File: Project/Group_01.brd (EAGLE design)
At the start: 71.1 x 54.3 mm, 29 parts, among them J1 POWER_JACKPTH_LOCK, U1 +12v, U4 TMUX1208

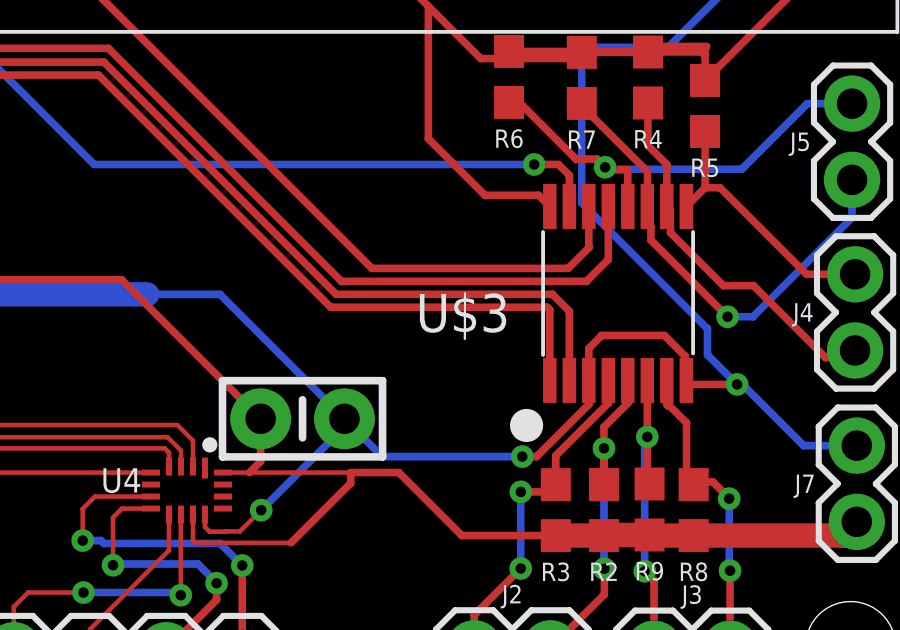
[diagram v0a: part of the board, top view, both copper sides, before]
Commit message: Changed name
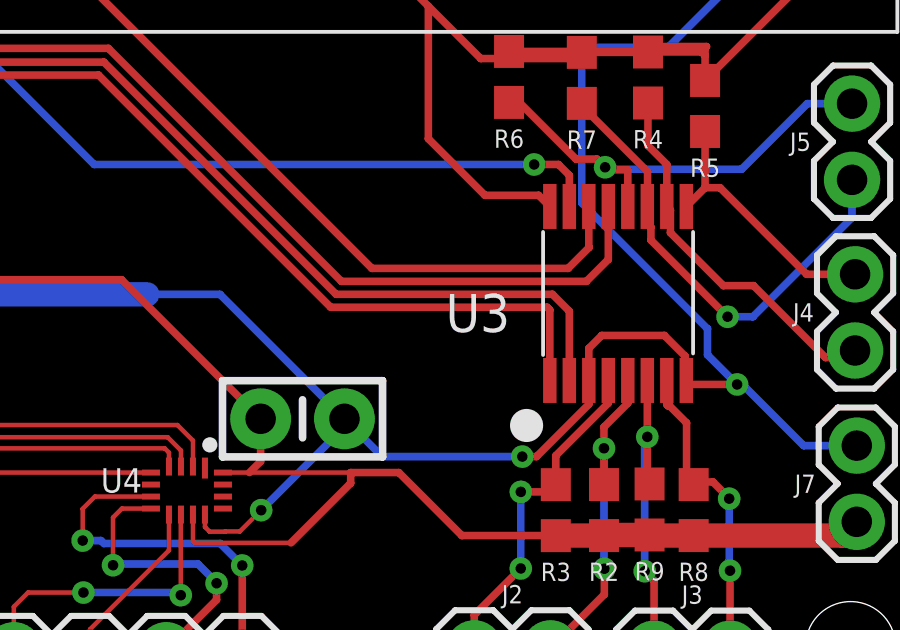
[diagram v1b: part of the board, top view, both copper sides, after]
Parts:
- renumbered U$3 to U3
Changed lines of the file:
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@@
 <attribute name="VALUE" x="41.13478125" y="50.174271875" size="0.6096" layer="27" font="vector" ratio="20" rot="R90" align="top-center"/>
 </element>
-<element name="U$3" library="Group_01_Library" package="TSSOP16" value="TCA9546A" x="60.95" y="14.32" smashed="yes" rot="R90">
+<element name="U3" library="Group_01_Library" package="TSSOP16" value="TCA9546A" x="60.95" y="14.32" smashed="yes" rot="R90">
 <attribute name="NAME" x="57.347734375" y="13.668865625" size="1.27" layer="25" align="center-right"/>
 </element>
@@
 <contactref element="C1" pad="2"/>
 <contactref element="U1" pad="3"/>
-<contactref element="U$3" pad="8"/>
-<contactref element="U$3" pad="3"/>
+<contactref element="U3" pad="8"/>
+<contactref element="U3" pad="3"/>
 <contactref element="U$2" pad="28"/>
 <contactref element="R1" pad="P$1"/>
@@
 <contactref element="U1" pad="2"/>
 <contactref element="C1" pad="1"/>
-<contactref element="U$3" pad="16"/>
+<contactref element="U3" pad="16"/>
 <contactref element="R2" pad="2"/>
 <contactref element="R3" pad="2"/>
@@
 </signal>
 <signal name="I2C_SCL_0">
-<contactref element="U$3" pad="5"/>
+<contactref element="U3" pad="5"/>
 <contactref element="R2" pad="1"/>
 <contactref element="J2" pad="2"/>
@@
 <signal name="I2C_SDA_0">
 <contactref element="R3" pad="1"/>
-<contactref element="U$3" pad="4"/>
+<contactref element="U3" pad="4"/>
 <contactref element="J2" pad="1"/>
 <wire x1="60.625" y1="11.42" x2="60.625" y2="10.66395" width="0.254" layer="1"/>
@@
 </signal>
 <signal name="I2C_SDA_1">
-<contactref element="U$3" pad="6"/>
+<contactref element="U3" pad="6"/>
 <contactref element="R9" pad="1"/>
 <contactref element="J3" pad="1"/>
@@
 <signal name="I2C_SCL_1">
 <contactref element="R8" pad="1"/>
-<contactref element="U$3" pad="7"/>
+<contactref element="U3" pad="7"/>
 <contactref element="J3" pad="2"/>
 <wire x1="63.47" y1="7.95" x2="63.2333" y2="8.1867" width="0.254" layer="1"/>
@@
 </signal>
 <signal name="I2C_SDA_2">
-<contactref element="U$3" pad="9"/>
+<contactref element="U3" pad="9"/>
 <contactref element="R5" pad="1"/>
 <contactref element="J4" pad="1"/>
@@
 <signal name="I2C_SCL_2">
 <contactref element="R4" pad="1"/>
-<contactref element="U$3" pad="10"/>
+<contactref element="U3" pad="10"/>
 <contactref element="J4" pad="2"/>
 <wire x1="61.946959375" y1="20.669490625" x2="61.946959375" y2="19.24795" width="0.254" layer="1"/>
@@
 </signal>
 <signal name="I2C_SCL_3">
-<contactref element="U$3" pad="12"/>
+<contactref element="U3" pad="12"/>
 <contactref element="R6" pad="1"/>
 <contactref element="J5" pad="2"/>
@@
 </signal>
 <signal name="I2C_SDA_3">
-<contactref element="U$3" pad="11"/>
+<contactref element="U3" pad="11"/>
 <contactref element="R7" pad="1"/>
 <contactref element="J5" pad="1"/>
@@
 </signal>
 <signal name="I2C_SDA">
-<contactref element="U$3" pad="15"/>
+<contactref element="U3" pad="15"/>
 <contactref element="U$2" pad="15"/>
 <wire x1="59.325" y1="17.22" x2="59.324240625" y2="17.220759375" width="0.254" layer="1"/>
@@
 </signal>
 <signal name="I2C_SCL">
-<contactref element="U$3" pad="14"/>
+<contactref element="U3" pad="14"/>
 <contactref element="U$2" pad="16"/>
 <wire x1="59.975" y1="17.22" x2="59.975" y2="15.866859375" width="0.254" layer="1"/>
@@
 </signal>
 <signal name="I2C_A2">
-<contactref element="U$3" pad="13"/>
+<contactref element="U3" pad="13"/>
 <contactref element="U$2" pad="8"/>
 <wire x1="60.625" y1="17.22" x2="60.625" y2="15.45490625" width="0.254" layer="1"/>
@@
 </signal>
 <signal name="I2C_A1">
-<contactref element="U$3" pad="2"/>
+<contactref element="U3" pad="2"/>
 <contactref element="U$2" pad="7"/>
 <wire x1="59.325" y1="11.42" x2="59.325" y2="13.730478125" width="0.254" layer="1"/>
@@
 </signal>
 <signal name="I2C_A0">
-<contactref element="U$3" pad="1"/>
+<contactref element="U3" pad="1"/>
 <contactref element="U$2" pad="6"/>
 <wire x1="58.675" y1="11.42" x2="58.675" y2="13.76981875" width="0.254" layer="1"/>

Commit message: Revert "Changed name"
This reverts commit 609342ddda2755176251b6021189b0587eea2b8d.
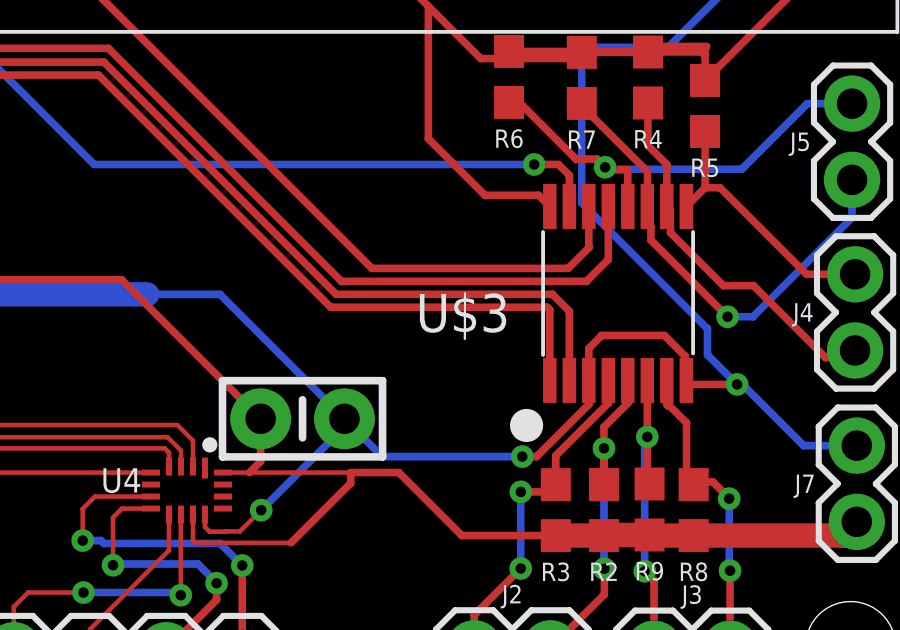
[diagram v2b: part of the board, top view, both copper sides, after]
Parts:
- renumbered U3 to U$3
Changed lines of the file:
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@@
 <attribute name="VALUE" x="41.13478125" y="50.174271875" size="0.6096" layer="27" font="vector" ratio="20" rot="R90" align="top-center"/>
 </element>
-<element name="U3" library="Group_01_Library" package="TSSOP16" value="TCA9546A" x="60.95" y="14.32" smashed="yes" rot="R90">
+<element name="U$3" library="Group_01_Library" package="TSSOP16" value="TCA9546A" x="60.95" y="14.32" smashed="yes" rot="R90">
 <attribute name="NAME" x="57.347734375" y="13.668865625" size="1.27" layer="25" align="center-right"/>
 </element>
@@
 <contactref element="C1" pad="2"/>
 <contactref element="U1" pad="3"/>
-<contactref element="U3" pad="8"/>
-<contactref element="U3" pad="3"/>
+<contactref element="U$3" pad="8"/>
+<contactref element="U$3" pad="3"/>
 <contactref element="U$2" pad="28"/>
 <contactref element="R1" pad="P$1"/>
@@
 <contactref element="U1" pad="2"/>
 <contactref element="C1" pad="1"/>
-<contactref element="U3" pad="16"/>
+<contactref element="U$3" pad="16"/>
 <contactref element="R2" pad="2"/>
 <contactref element="R3" pad="2"/>
@@
 </signal>
 <signal name="I2C_SCL_0">
-<contactref element="U3" pad="5"/>
+<contactref element="U$3" pad="5"/>
 <contactref element="R2" pad="1"/>
 <contactref element="J2" pad="2"/>
@@
 <signal name="I2C_SDA_0">
 <contactref element="R3" pad="1"/>
-<contactref element="U3" pad="4"/>
+<contactref element="U$3" pad="4"/>
 <contactref element="J2" pad="1"/>
 <wire x1="60.625" y1="11.42" x2="60.625" y2="10.66395" width="0.254" layer="1"/>
@@
 </signal>
 <signal name="I2C_SDA_1">
-<contactref element="U3" pad="6"/>
+<contactref element="U$3" pad="6"/>
 <contactref element="R9" pad="1"/>
 <contactref element="J3" pad="1"/>
@@
 <signal name="I2C_SCL_1">
 <contactref element="R8" pad="1"/>
-<contactref element="U3" pad="7"/>
+<contactref element="U$3" pad="7"/>
 <contactref element="J3" pad="2"/>
 <wire x1="63.47" y1="7.95" x2="63.2333" y2="8.1867" width="0.254" layer="1"/>
@@
 </signal>
 <signal name="I2C_SDA_2">
-<contactref element="U3" pad="9"/>
+<contactref element="U$3" pad="9"/>
 <contactref element="R5" pad="1"/>
 <contactref element="J4" pad="1"/>
@@
 <signal name="I2C_SCL_2">
 <contactref element="R4" pad="1"/>
-<contactref element="U3" pad="10"/>
+<contactref element="U$3" pad="10"/>
 <contactref element="J4" pad="2"/>
 <wire x1="61.946959375" y1="20.669490625" x2="61.946959375" y2="19.24795" width="0.254" layer="1"/>
@@
 </signal>
 <signal name="I2C_SCL_3">
-<contactref element="U3" pad="12"/>
+<contactref element="U$3" pad="12"/>
 <contactref element="R6" pad="1"/>
 <contactref element="J5" pad="2"/>
@@
 </signal>
 <signal name="I2C_SDA_3">
-<contactref element="U3" pad="11"/>
+<contactref element="U$3" pad="11"/>
 <contactref element="R7" pad="1"/>
 <contactref element="J5" pad="1"/>
@@
 </signal>
 <signal name="I2C_SDA">
-<contactref element="U3" pad="15"/>
+<contactref element="U$3" pad="15"/>
 <contactref element="U$2" pad="15"/>
 <wire x1="59.325" y1="17.22" x2="59.324240625" y2="17.220759375" width="0.254" layer="1"/>
@@
 </signal>
 <signal name="I2C_SCL">
-<contactref element="U3" pad="14"/>
+<contactref element="U$3" pad="14"/>
 <contactref element="U$2" pad="16"/>
 <wire x1="59.975" y1="17.22" x2="59.975" y2="15.866859375" width="0.254" layer="1"/>
@@
 </signal>
 <signal name="I2C_A2">
-<contactref element="U3" pad="13"/>
+<contactref element="U$3" pad="13"/>
 <contactref element="U$2" pad="8"/>
 <wire x1="60.625" y1="17.22" x2="60.625" y2="15.45490625" width="0.254" layer="1"/>
@@
 </signal>
 <signal name="I2C_A1">
-<contactref element="U3" pad="2"/>
+<contactref element="U$3" pad="2"/>
 <contactref element="U$2" pad="7"/>
 <wire x1="59.325" y1="11.42" x2="59.325" y2="13.730478125" width="0.254" layer="1"/>
@@
 </signal>
 <signal name="I2C_A0">
-<contactref element="U3" pad="1"/>
+<contactref element="U$3" pad="1"/>
 <contactref element="U$2" pad="6"/>
 <wire x1="58.675" y1="11.42" x2="58.675" y2="13.76981875" width="0.254" layer="1"/>
